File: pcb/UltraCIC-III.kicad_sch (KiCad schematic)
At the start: 4 parts, among them J1 Conn_01x08, J2 Conn_01x08, U1 ATtiny25-20S, U2 ATtiny25-20P

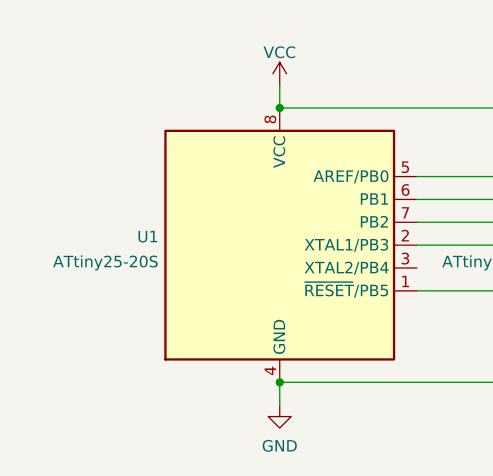
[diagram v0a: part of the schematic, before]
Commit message: Updated PCB
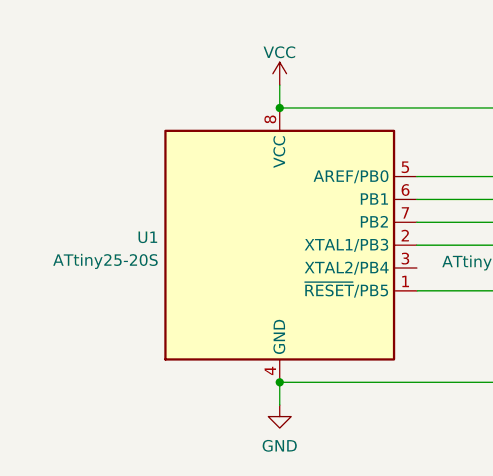
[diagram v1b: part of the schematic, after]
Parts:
- U1: footprint Package_SO:SOIC-8W_5.3x5.3mm_P1.27mm -> Eigene:SOP-8-Wide
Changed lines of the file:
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@@
   (symbol (lib_id "MCU_Microchip_ATtiny:ATtiny25-20S") (at 96.52 78.74 0) (unit 1)
     (in_bom yes) (on_board yes) (fields_autoplaced)
-    (property "Reference" "U1" (id 0) (at 83.0581 77.8315 0)
+    (property "Reference" "U1" (id 0) (at 83.0581 77.9053 0)
       (effects (font (size 1.27 1.27)) (justify right))
     )
-    (property "Value" "ATtiny25-20S" (id 1) (at 83.0581 80.6066 0)
+    (property "Value" "ATtiny25-20S" (id 1) (at 83.0581 80.4422 0)
       (effects (font (size 1.27 1.27)) (justify right))
     )
-    (property "Footprint" "Package_SO:SOIC-8W_5.3x5.3mm_P1.27mm" (id 2) (at 96.52 78.74 0)
+    (property "Footprint" "Eigene:SOP-8-Wide" (id 2) (at 96.52 78.74 0)
       (effects (font (size 1.27 1.27) italic) hide)
     )
@@
     )
     (path "/7f4e0710-12e3-446c-9fe8-f9b39e6a045f"
-      (reference "U1") (unit 1) (value "ATtiny25-20S") (footprint "Package_SO:SOIC-8W_5.3x5.3mm_P1.27mm")
+      (reference "U1") (unit 1) (value "ATtiny25-20S") (footprint "Eigene:SOP-8-Wide")
     )
     (path "/7f3f6f32-3ef3-4f5d-918e-5969cbea43e0"
